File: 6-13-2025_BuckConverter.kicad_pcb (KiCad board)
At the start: 2 copper layers, 45.5 x 28 mm, 17 parts, among them J1 6V to 35V, J2 5V 3A, U1 MP2338GTL-Z

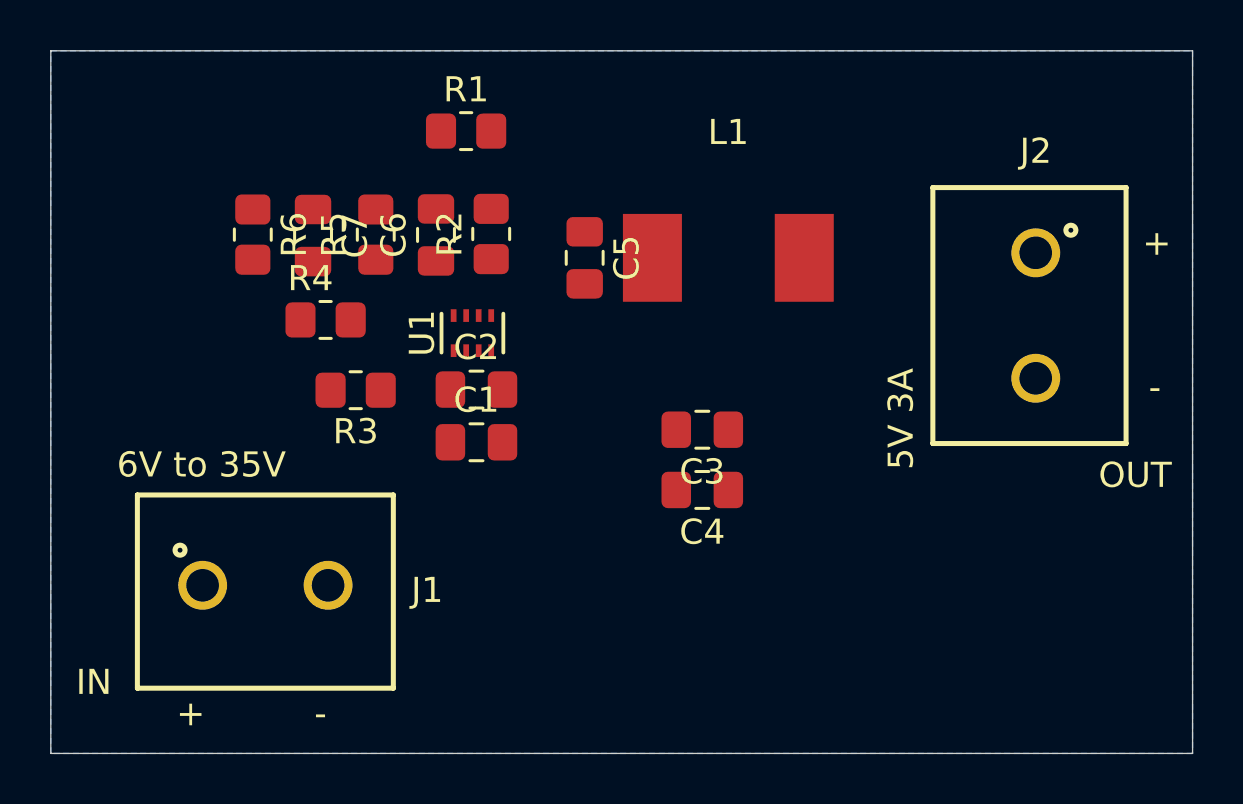
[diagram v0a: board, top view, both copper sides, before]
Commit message: Completed PCB layout and routing.
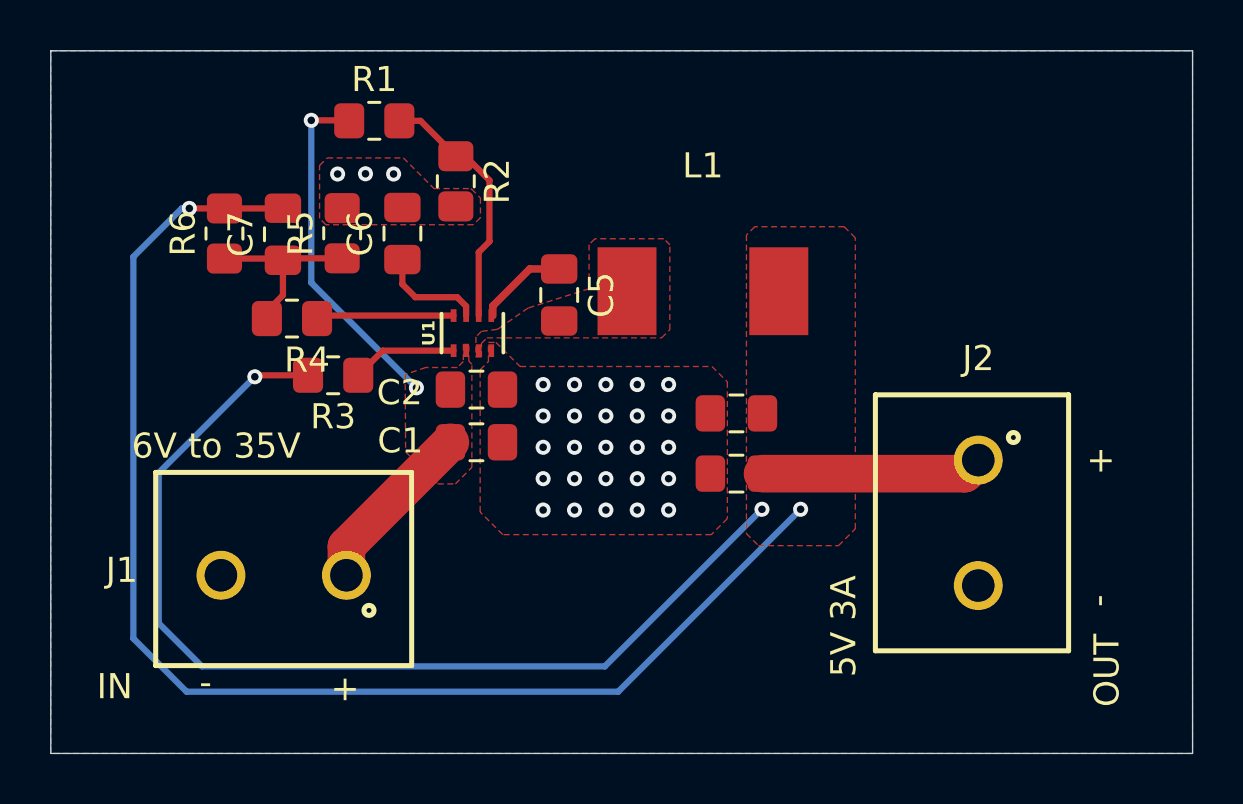
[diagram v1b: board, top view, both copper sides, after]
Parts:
- moved J2 8.57 mm to (158.2, 75.8)
- moved R1 3.68 mm to (134.1, 59.8)
- moved R2 2.53 mm to (137.4, 62.2), turned to -90 degrees
- moved C5 1.79 mm to (141.5, 66.7)
- moved L1 1.67 mm to (147.2, 66.6)
- moved C4 1.51 mm to (148.6, 73.8)
- moved C3 1.51 mm to (148.6, 71.5)
- moved C6 1.34 mm to (135.3, 64.3)
- moved R5 1.34 mm to (132.9, 64.3)
- moved R4 1.34 mm to (130.9, 67.7), turned to 180 degrees
- moved C7 1.20 mm to (130.5, 64.3), turned to 90 degrees
- moved R6 1.13 mm to (128.2, 64.3), turned to 90 degrees
- moved R3 1.08 mm to (132.5, 69.9)
- moved J1 0.83 mm to (130.5, 77.9), turned to 180 degrees
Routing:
- net Net-(J2-VIN): track 0.00 -> 102.2 mm, vias 0 -> 4
- net Net-(J1-VIN): track 0.00 -> 20.9 mm, vias 0 -> 2
- net Net-(U1-EN): track 0.00 -> 10.1 mm
- net Net-(C7-Pad1): track 0.00 -> 7.34 mm
- net Net-(U1-FB): track 0.00 -> 5.49 mm
- net Net-(U1-SS): track 0.00 -> 4.26 mm
- net Net-(U1-PG): track 0.00 -> 4.21 mm
- net Net-(U1-BST): track 0.00 -> 3.64 mm
- net GND: vias 0 -> 28
- added copper zone on F.Cu, net GND
- added copper zone on F.Cu, net Net-(J1-VIN)
- added copper zone on F.Cu, net Net-(J2-VIN)
- added copper zone on F.Cu, net Net-(U1-SW)
